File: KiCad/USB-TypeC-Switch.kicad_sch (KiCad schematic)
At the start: 9 parts, among them J1 USB_C_IN_1, J2 USB_C_IN_2, J3 USB_C_OUT

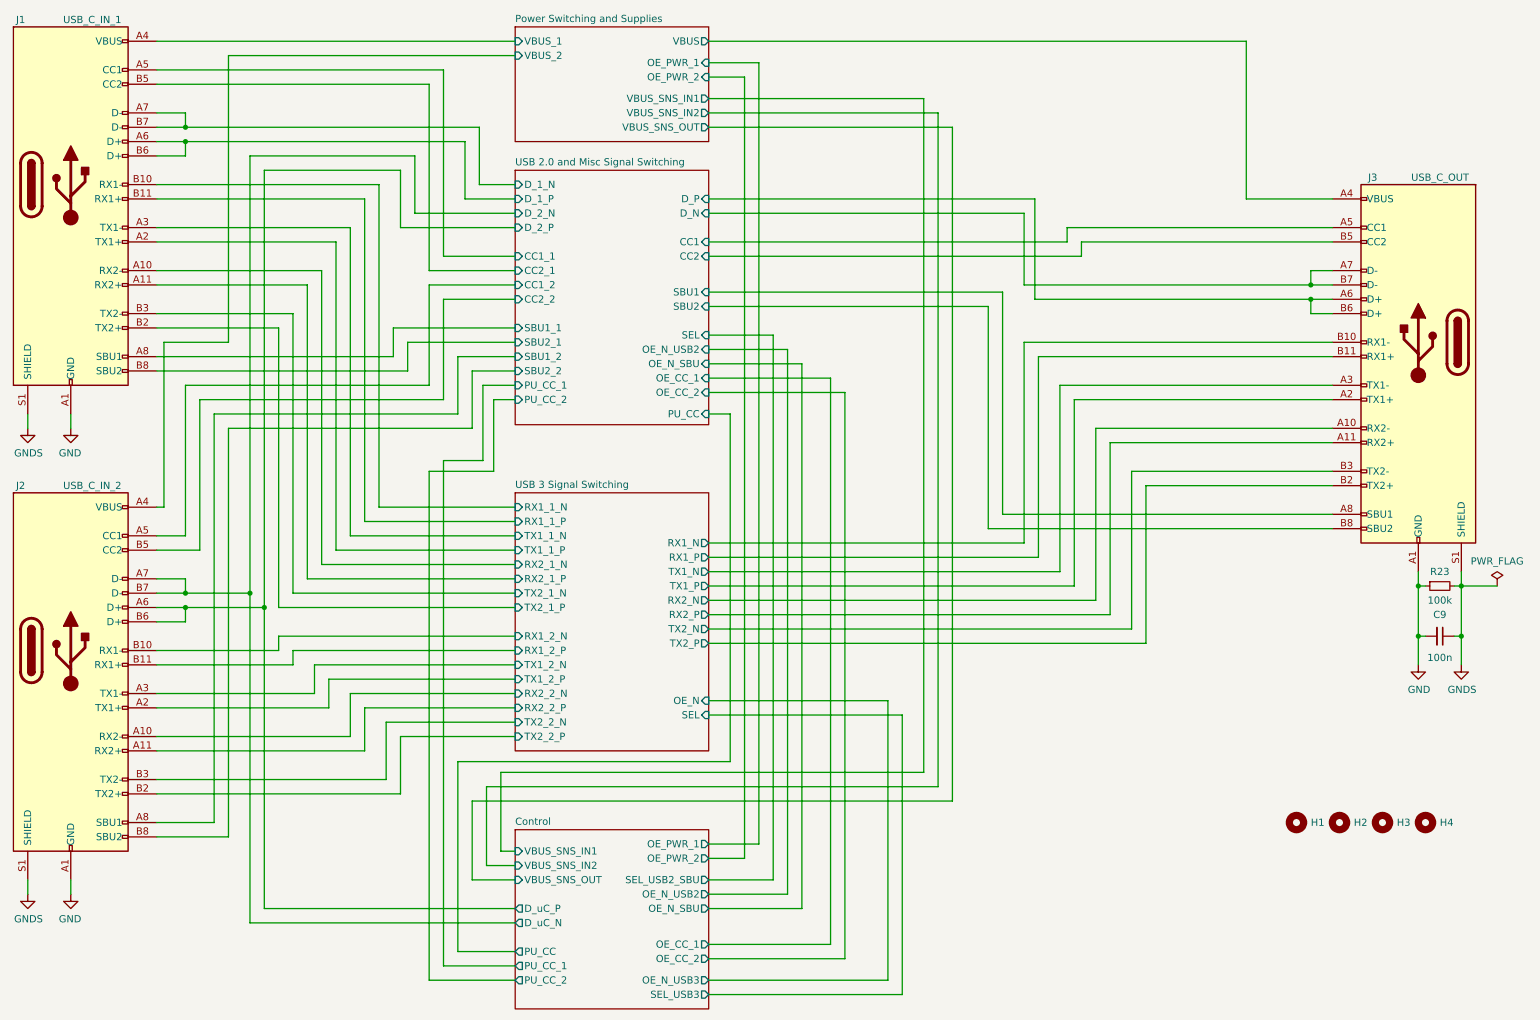
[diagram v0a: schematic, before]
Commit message: update footprints + render + power pull-ups
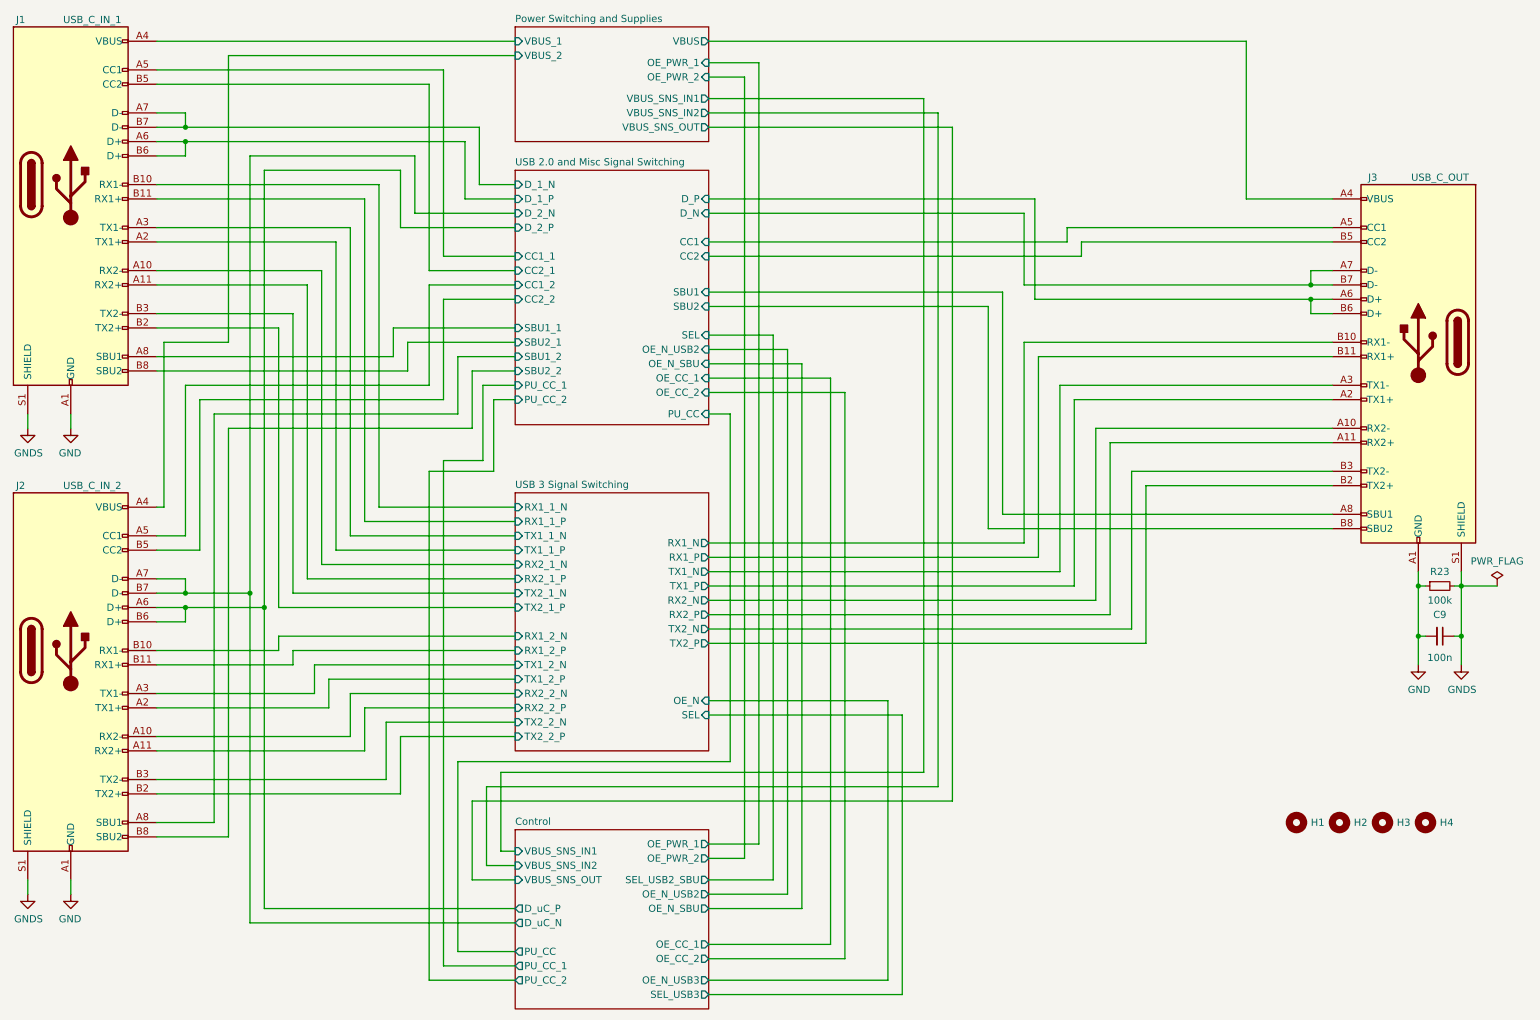
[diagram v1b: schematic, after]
